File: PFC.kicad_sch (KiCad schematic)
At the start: 42 parts, among them IC1 UCC28180D, J1 Conn_01x02_Pin, J2 Conn_01x02_Pin, J3 Conn_01x04_Pin, J4 Conn_01x02_Pin, Q1 IMBG120R234M2HXTMA1, Q2 T2N7002AK, Q3 T2N7002AK, U1 MGJ2D241505SC, U2 MGJ2D241505SC, U3 UCC21520DW, U4 L7805, U5 MCP6002-xSN, U6 MCP6567, U7 74AHC1G14, U8 EL817

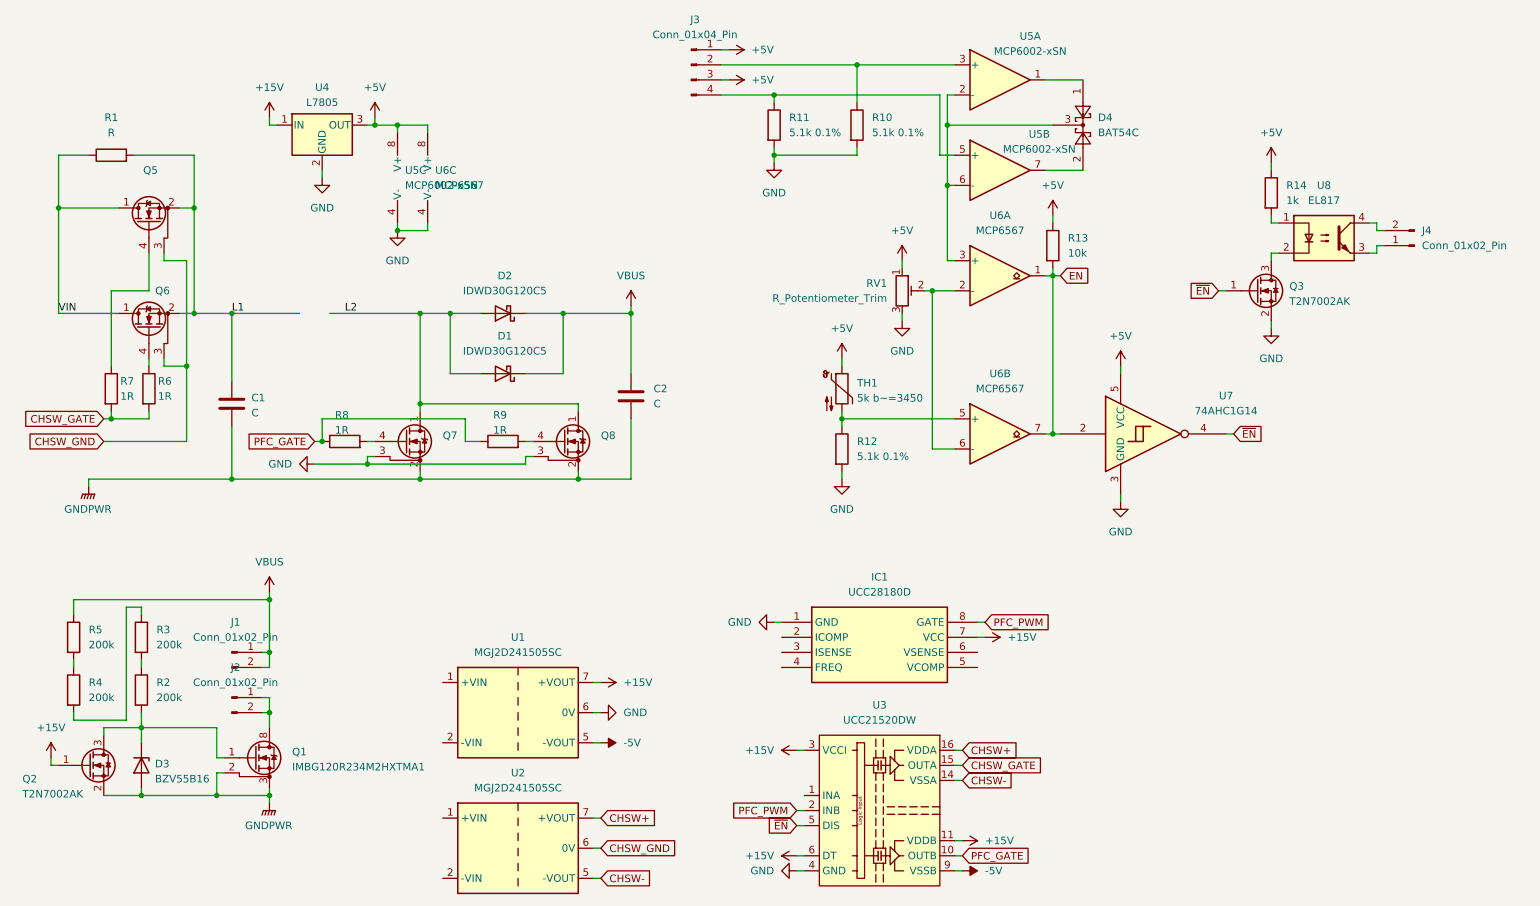
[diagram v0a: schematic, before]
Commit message: initial work
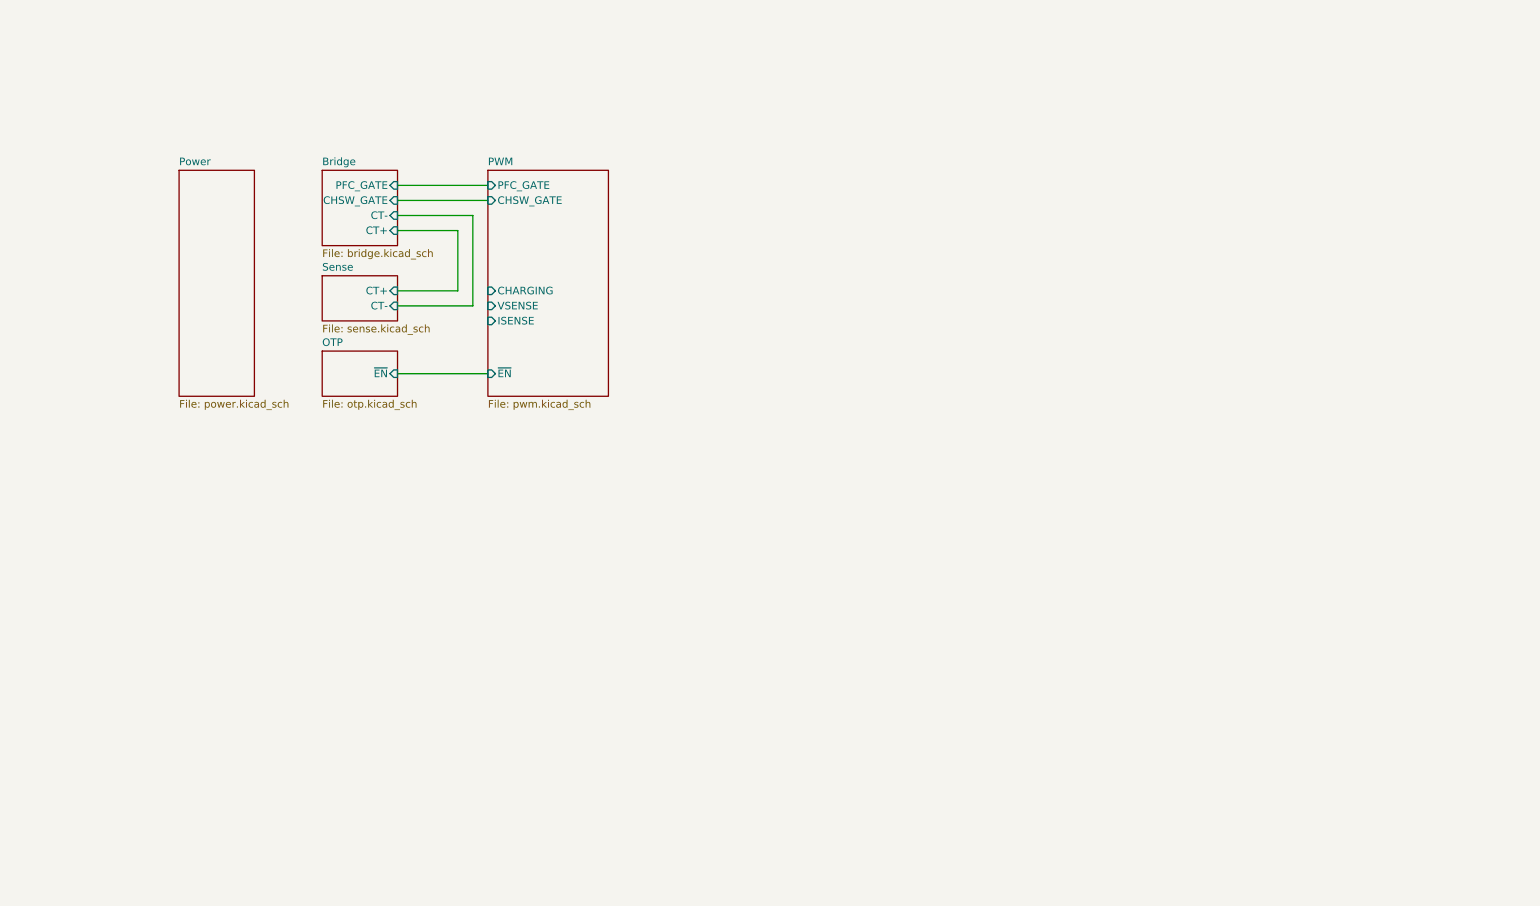
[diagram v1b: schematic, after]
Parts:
- removed C1, C2: C, symbol Device:C
- removed D1, D2: IDWD30G120C5, Package_TO_SOT_THT:TO-247-2_Horizontal_TabDown, symbol Diode:C4D20120H
- removed D3: BZV55B16, Diode_SMD:D_MiniMELF, symbol Diode:BZV55B16
- removed D4: BAT54C, Package_TO_SOT_SMD:SOT-23, symbol Diode:BAT54C
- removed IC1: UCC28180D, Package_SO:SOIC-8_3.9x4.9mm_P1.27mm, symbol New_Library:UCC28180D
- removed J1, J2, J4: Conn_01x02_Pin, Connector_Molex:Molex_KK-254_AE-6410-02A_1x02_P2.54mm_Vertical, symbol Connector:Conn_01x02_Pin
- removed J3: Conn_01x04_Pin, Connector_Molex:Molex_KK-254_AE-6410-04A_1x04_P2.54mm_Vertical, symbol Connector:Conn_01x04_Pin
- removed Q1: IMBG120R234M2HXTMA1, Package_TO_SOT_SMD:TO-263-7_TabPin8, symbol Transistor_FET:C2M1000170J
- removed Q2, Q3: T2N7002AK, Package_TO_SOT_SMD:SOT-23, symbol Transistor_FET:T2N7002AK
- removed Q5, Q6, Q7, Q8: (no value), Package_TO_SOT_THT:TO-247-4_Horizontal_TabDown, symbol Transistor_FET:C3M0030090K
- removed R1: R, symbol Device:R
- removed R10, R11, R12: 5.1k 0.1%, Resistor_SMD:R_0805_2012Metric, symbol Device:R
- removed R13: 10k, Resistor_SMD:R_0805_2012Metric, symbol Device:R
- removed R14: 1k, Resistor_SMD:R_0805_2012Metric, symbol Device:R
- removed R2, R3, R4, R5: 200k, Resistor_SMD:R_2512_6332Metric, symbol Device:R
- removed R6, R7, R8, R9: 1R, Resistor_SMD:R_0805_2012Metric, symbol Device:R
- removed RV1: R_Potentiometer_Trim, Potentiometer_THT:Potentiometer_Vishay_T93YA_Vertical, symbol Device:R_Potentiometer_Trim
- removed TH1: 5k b~=3450, Resistor_SMD:R_0805_2012Metric, symbol Device:Thermistor_NTC
- removed U1, U2: MGJ2D241505SC, Converter_DCDC:Converter_DCDC_Murata_MGJ2DxxxxxxSC_THT, symbol Converter_DCDC_Isolated:MGJ2D241505SC
- removed U3: UCC21520DW, Package_SO:SOIC-16W_7.5x10.3mm_P1.27mm, symbol Driver_FET:UCC21520DW
- removed U4: L7805, digikey-footprints:TO-252-3, symbol Regulator_Linear:L7805
- removed U5: MCP6002-xSN, Package_SO:SOIC-8_3.9x4.9mm_P1.27mm, symbol Amplifier_Operational:MCP6002-xSN
- removed U6: MCP6567, symbol Comparator:MCP6567
- removed U7: 74AHC1G14, Package_TO_SOT_SMD:SOT-23-5, symbol 74xGxx:74AHC1G14
- removed U8: EL817, Package_DIP:DIP-4_W7.62mm, symbol Isolator:EL817
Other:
- added sheet Bridge (bridge.kicad_sch)
- added sheet OTP (otp.kicad_sch)
- added sheet PWM (pwm.kicad_sch)
- added sheet Power (power.kicad_sch)
- added sheet Sense (sense.kicad_sch)
